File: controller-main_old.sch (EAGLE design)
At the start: 24 parts

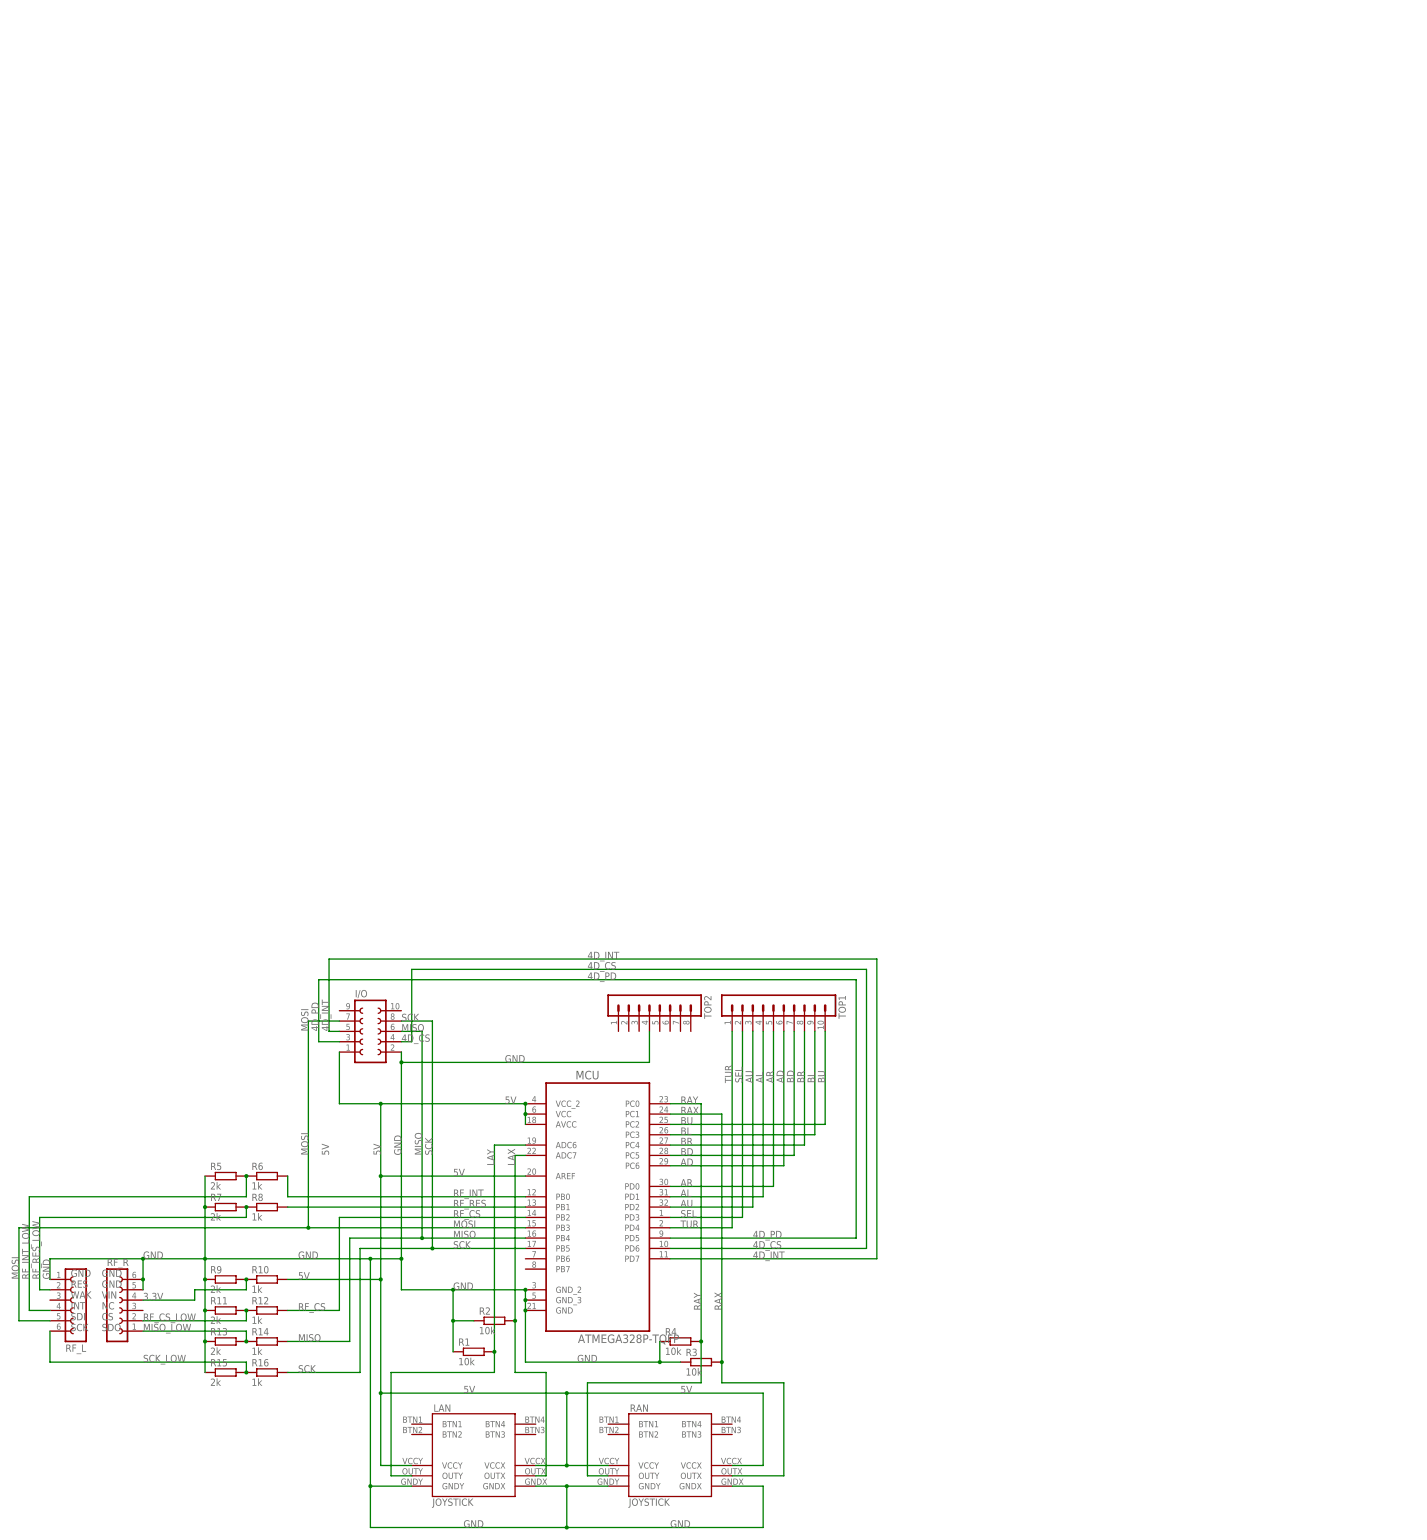
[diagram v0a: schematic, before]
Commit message: finished main board
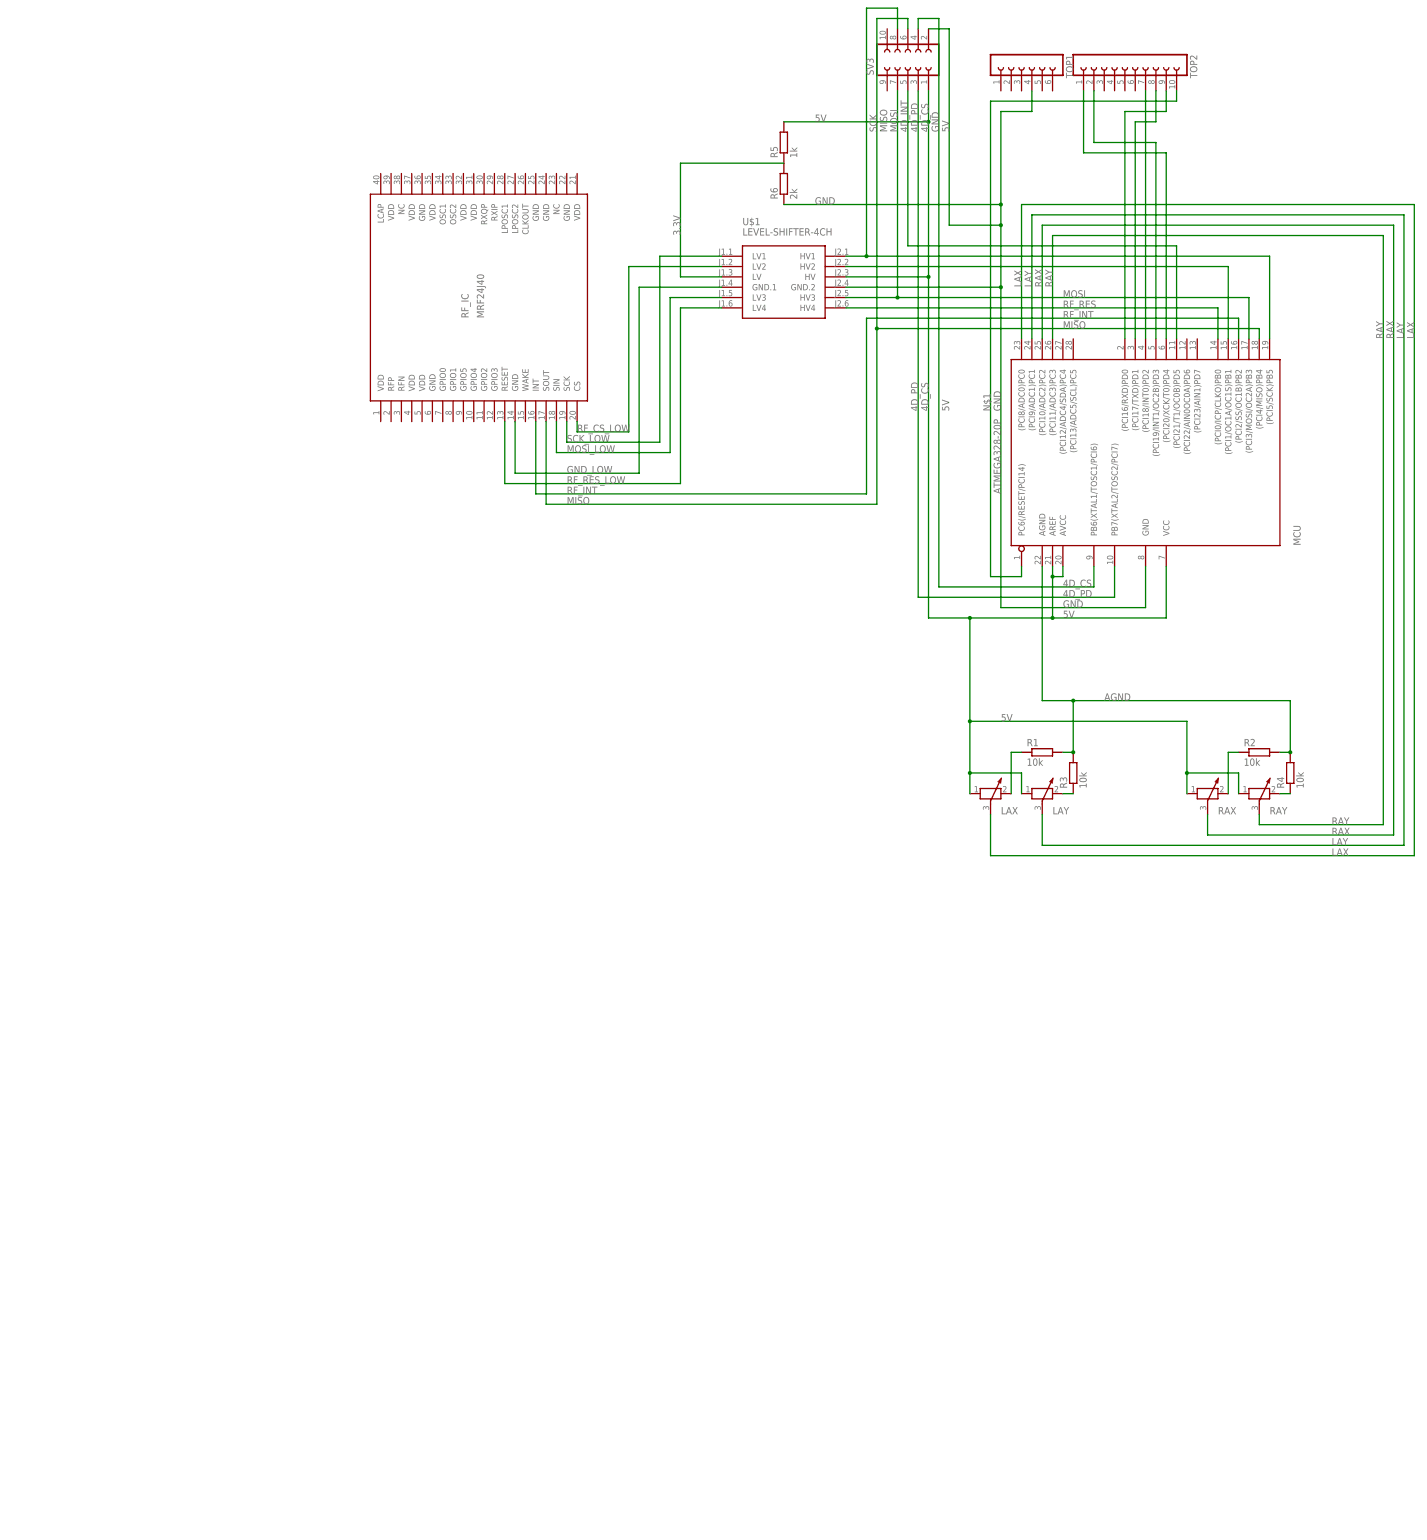
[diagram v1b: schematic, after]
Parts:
- removed I/O: (no value), con-lsta:FE05-2W
- removed LAN, RAN: JOYSTICK, joystick:JOYSTICKJOYSTICKWBTN
- removed R10, R12, R14, R16, R8: 1k, resistor:R-EU_M1206
- removed R11, R13, R15, R7, R9: 2k, resistor:R-EU_M1206
- removed RF_L, RF_R: (no value), con-lsta:FE06-1
- added LAX, LAY, RAX, RAY: (no value), rcl:POTENTIOMETER_PT-10S
- added RF_IC: MRF24J40, microchip:MRF24J40
- added SV3: (no value), con-lsta:FE05-2W
- added U$1: LEVEL-SHIFTER-4CH, diy-modules:LEVEL-SHIFTER-4CH
- MCU: value ATMEGA328P-TQFP -> ATMEGA328-20P; device Atmel_By_element14_Batch_1-00:ATMEGA328P-AU -> atmega328p:ATMEGA328-20P
- R1, R2, R3, R4: device resistor:R-EU_M1206 -> rcl:R-EU_0204/5
- R5: value 2k -> 1k; device resistor:R-EU_M1206 -> rcl:R-EU_0204/5
- R6: value 1k -> 2k; device resistor:R-EU_M1206 -> rcl:R-EU_0204/5
- TOP1: device con-lstb:MA10-1W -> con-lsta:FE06W
- TOP2: device con-lstb:MA08-1 -> con-lsta:FE10W
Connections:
- removed net AD: MCU.PC6, TOP1.6
- removed net AL: MCU.PD1, TOP1.4
- removed net AR: MCU.PD0, TOP1.5
- removed net AU: MCU.PD2, TOP1.3
- removed net BD: MCU.PC5, TOP1.7
- removed net BL: MCU.PC3, TOP1.9
- removed net BR: MCU.PC4, TOP1.8
- removed net BU: MCU.PC2, TOP1.10
- removed net MISO_LOW: R13.2, R14.1, RF_R.1
- removed net RF_INT_LOW: R5.2, R6.1, RF_L.4
- removed net SEL: MCU.PD3, TOP1.2
- removed net TUR: MCU.PD4, TOP1.1
- new net AGND: MCU.AGND, R1.2, R2.2, R3.2, R4.2
- new net AGND1: LAX.2, R1.1
- new net AGND2: R2.1, RAX.2
- new net GND_LOW: RF_IC.GND@1, U$1.GND.1
- new net MOSI_LOW: RF_IC.SIN, U$1.LV3
- new net N$1: MCU.PC6(/RESET/PCI14), TOP2.10
- new net N$12: LAY.2, R3.1
- new net N$16: R4.1, RAY.2
- new net N$2: MCU.(PCI20/XCK/T0)PD4, TOP2.1
- new net N$3: MCU.(PCI19/INT1/OC2B)PD3, TOP2.2
- new net N$4: MCU.(PCI16/RXD)PD0, TOP2.9
- new net N$5: MCU.(PCI17/TXD)PD1, TOP2.8
- new net N$6: MCU.(PCI18/INT0)PD2, TOP2.7
- net 3.3V: now also R5.1, U$1.LV; no longer R10.1, R9.2, RF_R.4
- net 4D_CS: now also MCU.PB6(XTAL1/TOSC1/PCI6), SV3.4; no longer I/O.4, MCU.PD6
- net 4D_INT: now also MCU.(PCI21/T1/OC0B)PD5, SV3.5; no longer I/O.5, MCU.PD7
- net 4D_PD: now also MCU.PB7(XTAL2/TOSC2/PCI7), SV3.3; no longer I/O.3, MCU.PD5
- net 5V: now also LAX.1, LAY.1, R5.2, RAX.1, RAY.1, SV3.1, U$1.HV; no longer I/O.1, LAN.VCCX, LAN.VCCY, MCU.VCC_2, R10.2, RAN.VCCX, RAN.VCCY
- net GND: now also R6.1, SV3.2, TOP1.4, U$1.GND.2; no longer I/O.2, LAN.GNDX, LAN.GNDY, MCU.GND_2, MCU.GND_3, R1.1, R11.1, R13.1, R15.1, R2.1, R3.1, R4.1, R5.1, R7.1, R9.1, RAN.GNDX, RAN.GNDY, RF_L.1, RF_R.5, RF_R.6, TOP2.4
- net LAX: now also LAX.3, MCU.(PCI8/ADC0)PC0; no longer LAN.OUTX, MCU.ADC7, R2.2
- net LAY: now also LAY.3, MCU.(PCI9/ADC1)PC1; no longer LAN.OUTY, MCU.ADC6, R1.2
- net MISO: now also MCU.(PCI4/MISO)PB4, RF_IC.SOUT, SV3.6; no longer I/O.6, MCU.PB4, R14.2
- net MOSI: now also MCU.(PCI3/MOSI/OC2A)PB3, SV3.7, U$1.HV3; no longer I/O.7, MCU.PB3, RF_L.5
- net RAX: now also MCU.(PCI10/ADC2)PC2, RAX.3; no longer MCU.PC1, R3.2, RAN.OUTX
- net RAY: now also MCU.(PCI11/ADC3)PC3, RAY.3; no longer MCU.PC0, R4.2, RAN.OUTY
- net RF_CS: now also MCU.(PCI1/OC1A/OC1S)PB1, U$1.HV2; no longer MCU.PB2, R12.2
- net RF_CS_LOW: now also RF_IC.CS, U$1.LV2; no longer R11.2, R12.1, RF_R.2
- net RF_INT: now also MCU.(PCI2/SS/OC1B)PB2, RF_IC.INT; no longer MCU.PB0, R6.2
- net RF_RES: now also MCU.(PCI0/ICP/CLKO)PB0, U$1.HV4; no longer MCU.PB1, R8.2
- net RF_RES_LOW: now also RF_IC.RESET, U$1.LV4; no longer R7.2, R8.1, RF_L.2
- net SCK: now also MCU.(PCI5/SCK)PB5, SV3.8, U$1.HV1; no longer I/O.8, MCU.PB5, R16.2
- net SCK_LOW: now also RF_IC.SCK, U$1.LV1; no longer R15.2, R16.1, RF_L.6
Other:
- note removed: "GND GND VIN NC CS SDO"
- note removed: "GND RES WAK INT SDI SCK"
- moved on the sheet: R1, R2, R3, R4, R5, R6
